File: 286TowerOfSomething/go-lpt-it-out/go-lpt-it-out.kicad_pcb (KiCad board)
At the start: 2 copper layers, 45 parts, among them J1 Bus_ISA_8bit, J2 DE9, J3 Parallel, J4 Conn_02x05_Odd_Even, Q1 MMBT3904, SW1 SW_DIP_x06, SW2 SW_DIP_x07, U1 TL16C552A, U2 GD75232N, U3 GD75232N, U4 74LS138, U5 74LS138, U6 74HCU04, U7 74LS138, U9 74LS138, Y1 1.8432MHz

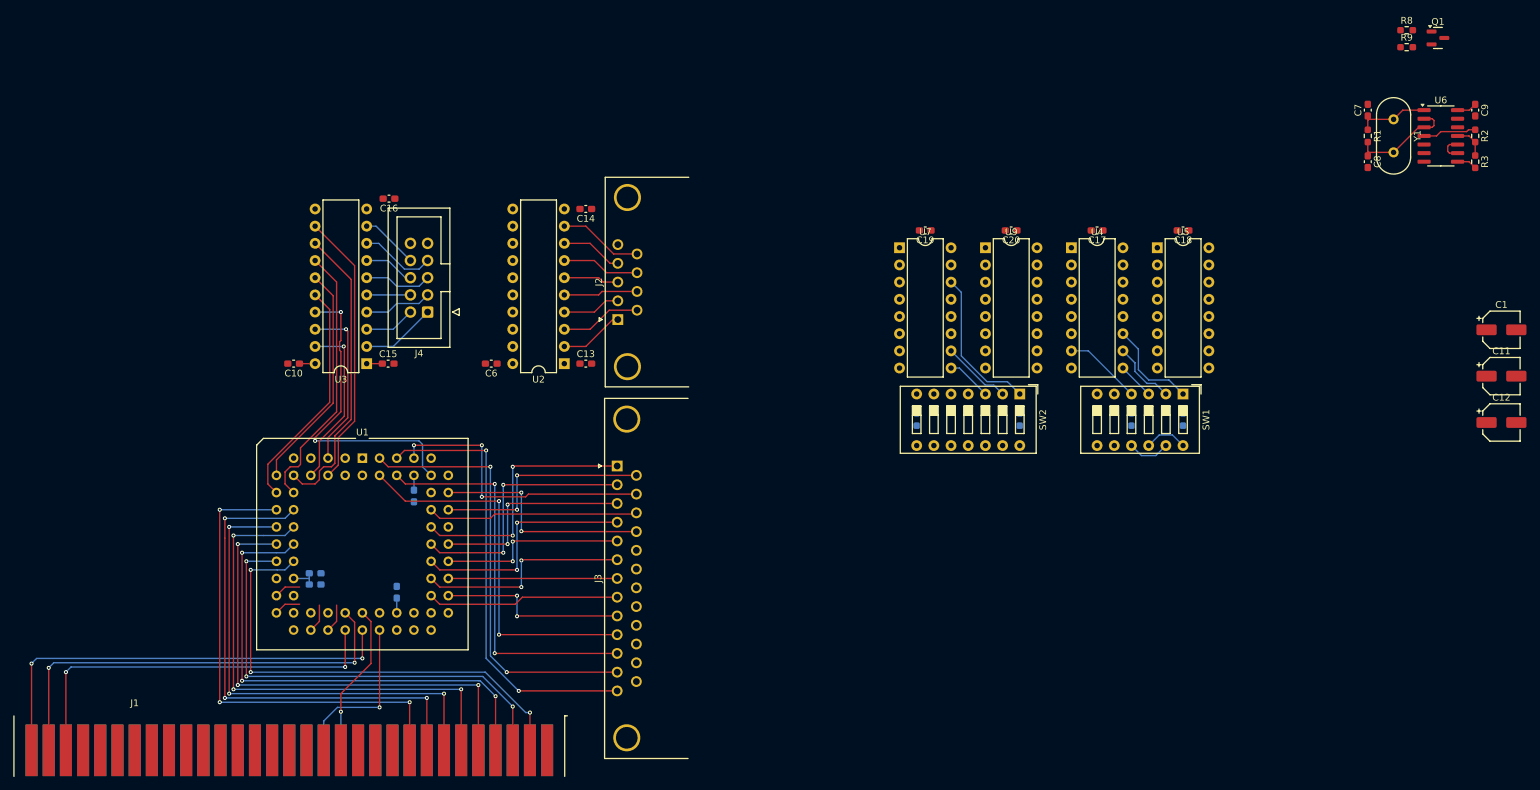
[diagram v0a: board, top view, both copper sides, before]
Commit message: More layout work on go-lpt-it-out
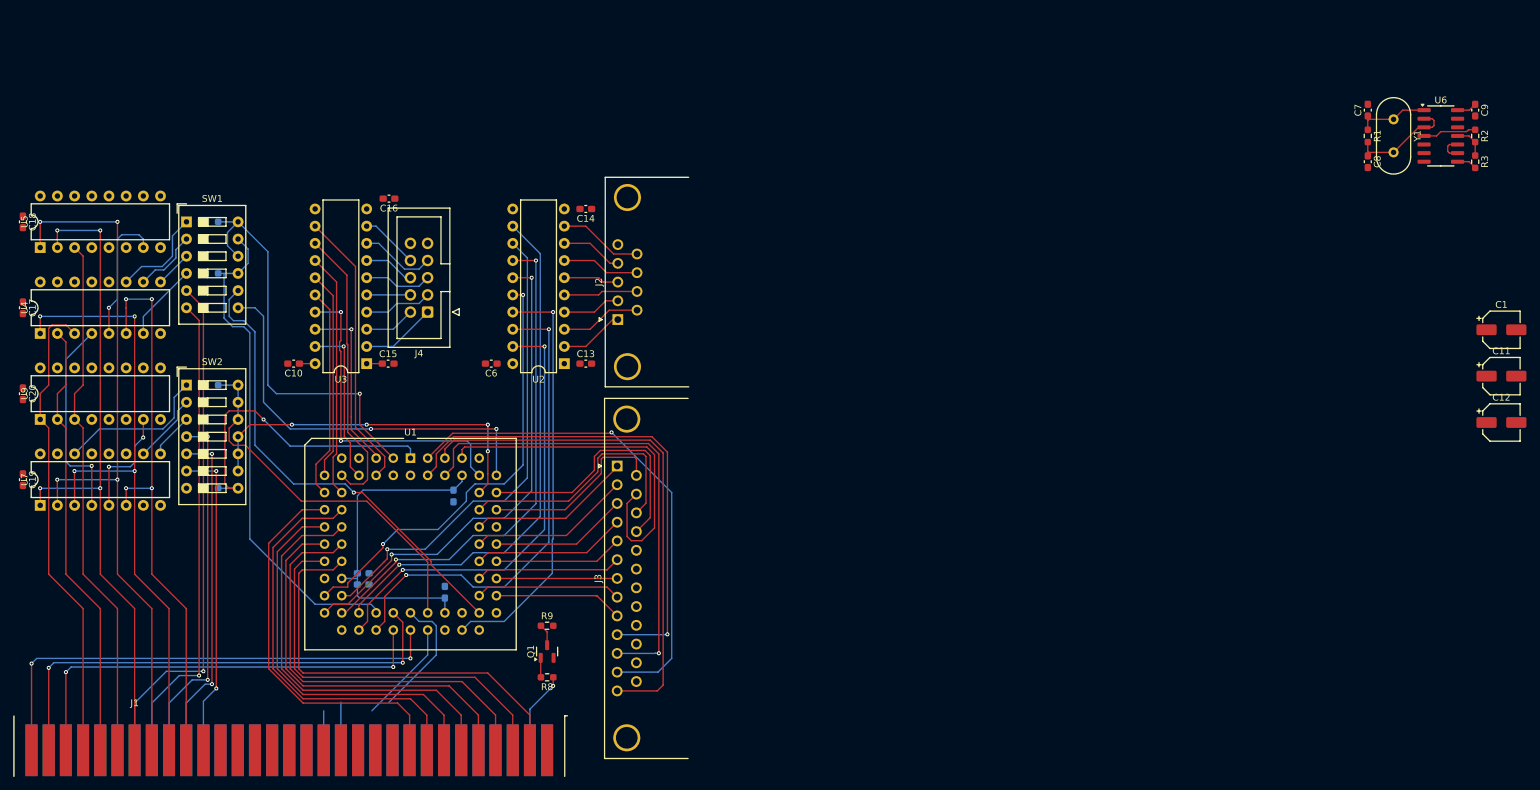
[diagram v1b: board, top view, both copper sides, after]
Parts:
- moved C18 171.5 mm to (44.5, 88.9), turned to -90 degrees
- moved U5 165.1 mm to (47.0, 92.7), turned to 90 degrees
- moved Q1 159.9 mm to (121.9, 152.4), turned to 90 degrees
- moved C17 159.2 mm to (44.5, 101.6), turned to -90 degrees
- moved R8 159.0 mm to (121.9, 156.2), turned to 180 degrees
- moved R9 153.1 mm to (121.9, 148.6)
- moved U4 152.9 mm to (47.0, 105.4), turned to 90 degrees
- moved SW1 149.5 mm to (68.6, 88.9), turned to 0 degrees
- moved C20 148.0 mm to (44.5, 114.3), turned to -90 degrees
- moved R6 146.5 mm to (72.4, 88.9), turned to 0 degrees
- moved U9 142.0 mm to (47.0, 118.1), turned to 90 degrees
- moved C19 138.3 mm to (44.5, 127.0), turned to -90 degrees
- moved R7 137.6 mm to (72.4, 96.5), turned to 0 degrees
- moved U7 132.6 mm to (47.0, 130.8), turned to 90 degrees
- moved SW2 123.2 mm to (68.6, 113.0), turned to 0 degrees
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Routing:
- net /Address and Config/A7: track 0.00 -> 108.1 mm, vias 0 -> 4
- net /Address and Config/A6: track 0.00 -> 99.3 mm, vias 0 -> 4
- net /Address and Config/A8: track 0.00 -> 96.7 mm, vias 0 -> 4
- net /Address and Config/A9: track 0.00 -> 84.0 mm, vias 0 -> 4
- net /Address and Config/A5: track 0.00 -> 78.0 mm
- net /~{UART0_RI}: track 0.00 -> 78.0 mm, vias 0 -> 1
- net /IRQ3: track 0.00 -> 76.4 mm, vias 0 -> 1
- net /~{UART0_CTS}: track 0.00 -> 75.0 mm, vias 0 -> 2
- net /~{UART0_DTR}: track 0.00 -> 71.0 mm, vias 0 -> 1
- net /IRQ4: track 0.00 -> 70.8 mm, vias 0 -> 1
- net /Address and Config/A3: track 0.00 -> 70.1 mm
- net /Address and Config/UART0_INT: track 0.00 -> 69.6 mm, vias 0 -> 1
- net /UART0_SOUT: track 3.96 -> 72.9 mm, vias 0 -> 2
- net /Address and Config/~{UART0_CS}: track 6.31 -> 74.5 mm
- net /~{UART0_DSR}: track 4.21 -> 71.4 mm, vias 0 -> 2
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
